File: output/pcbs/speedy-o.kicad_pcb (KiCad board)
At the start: 2 copper layers, 172 x 125.7 mm, 97 parts

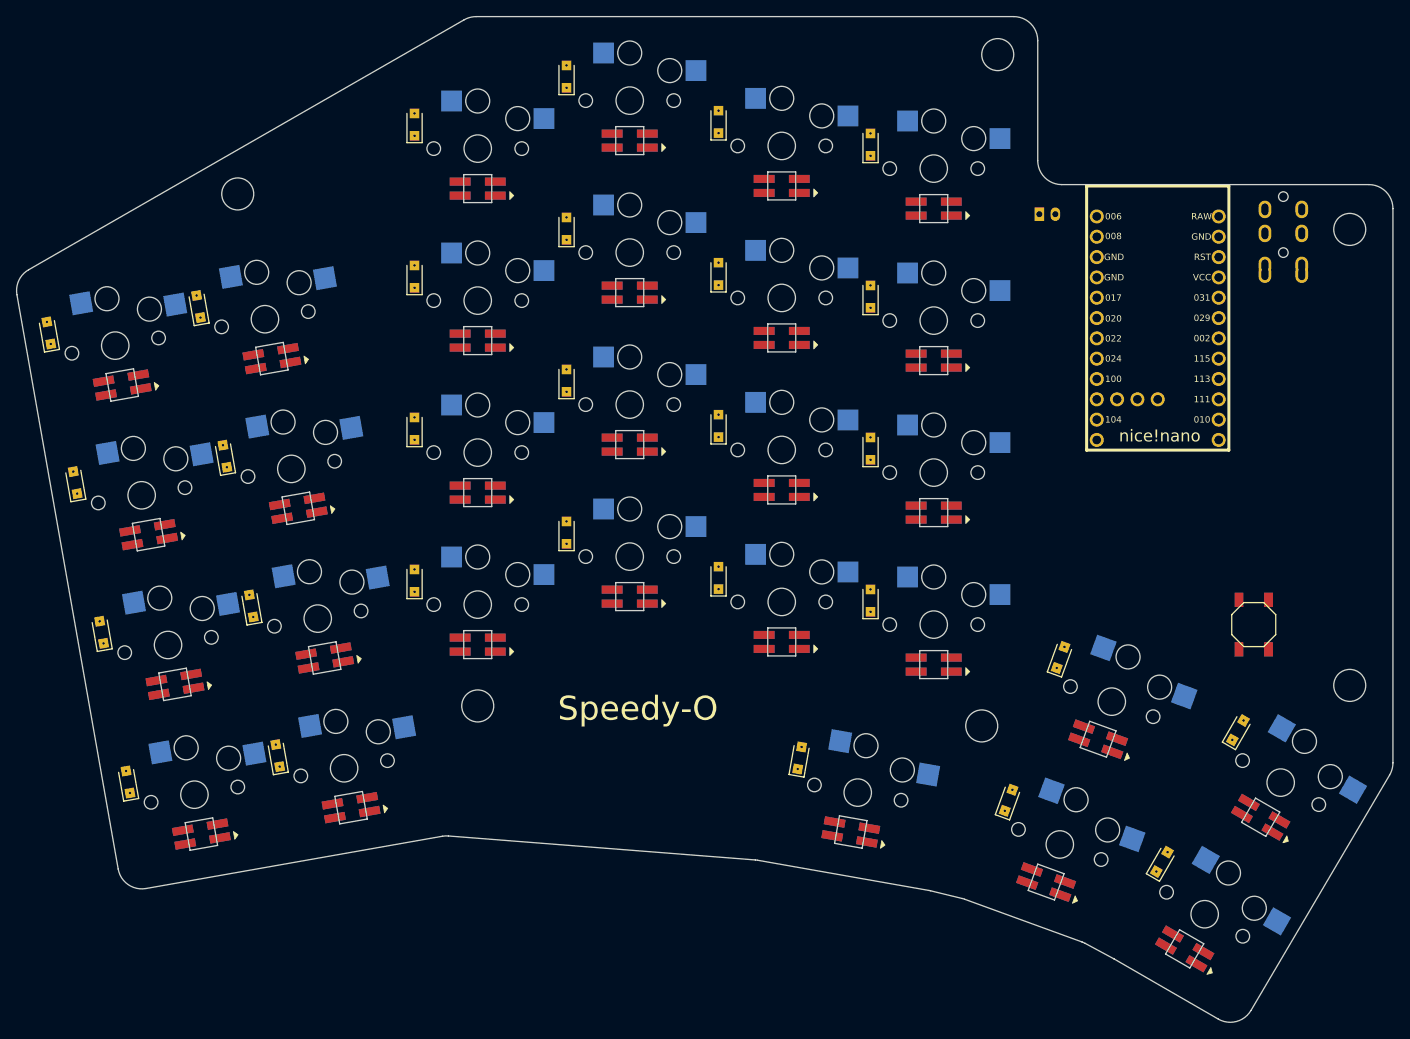
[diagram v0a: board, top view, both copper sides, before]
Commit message: update config
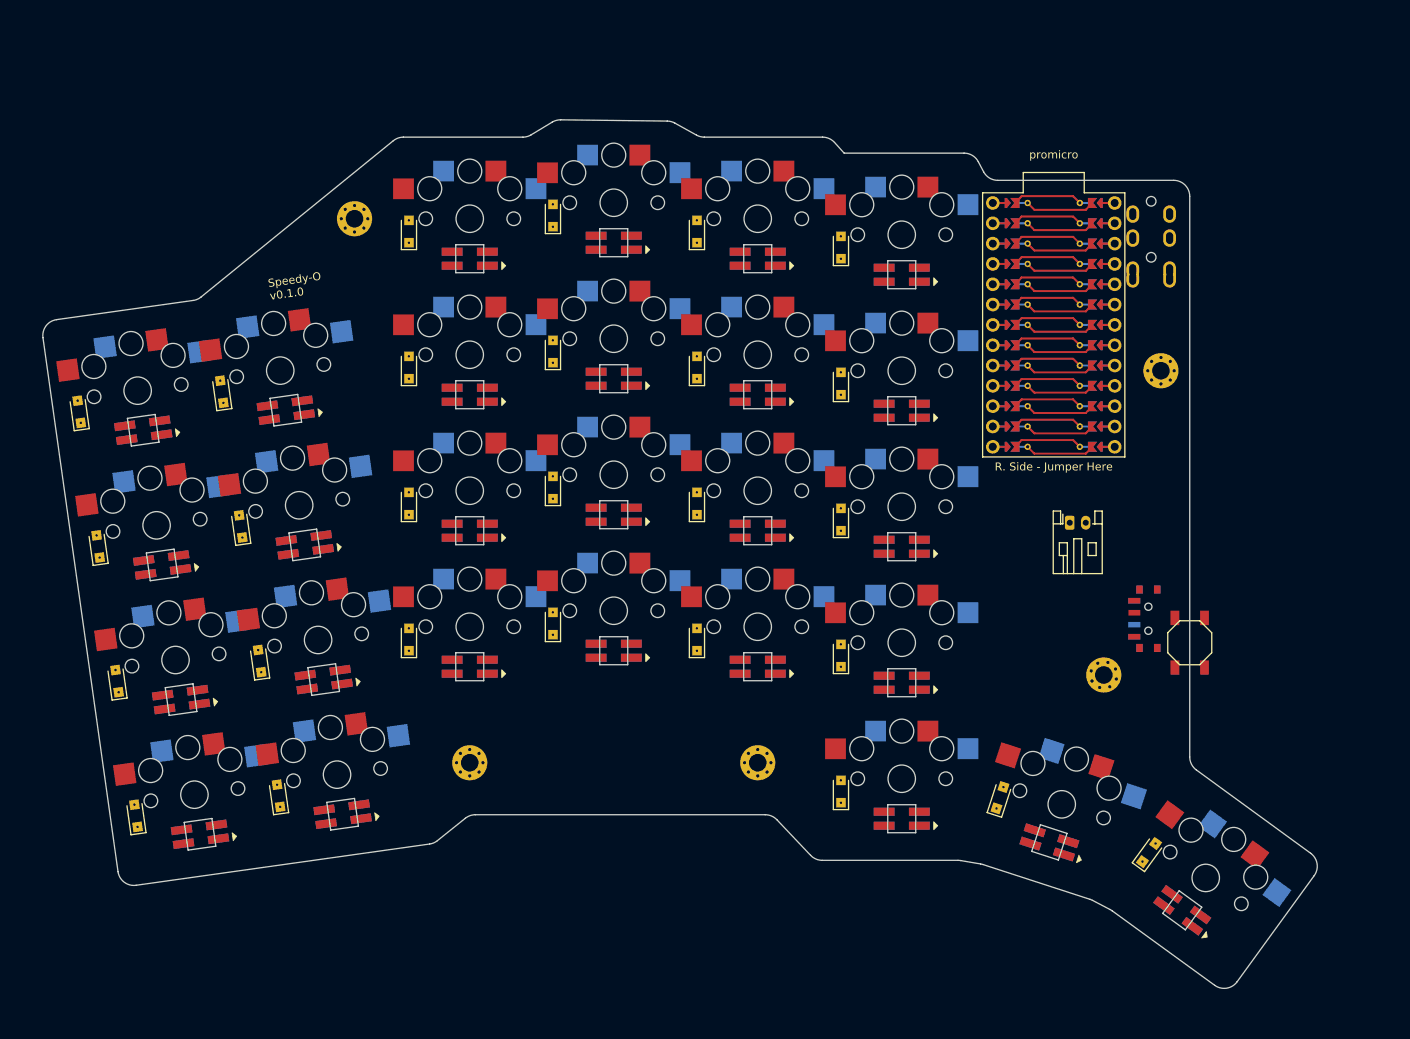
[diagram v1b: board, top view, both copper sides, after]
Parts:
- removed the ? at (135.4, 138.9)
- removed the ? at (198.4, 141.4)
- removed the ? at (244.4, 136.3)
- removed the ? at (105.4, 74.9)
- removed the ? at (200.4, 57.5)
- removed the ? at (244.4, 79.3)
- removed D28, D29: Nexperia_CFP3_SOD-123W, Diode_SMD:Nexperia_CFP3_SOD-123W
- removed JST1: , JST_PH_S2B-PH-K_02x2.00mm_Angled
- removed LED28, LED29: , WS2812B
- removed MCU1: nice_nano, nice_nano
- removed S28, S29: , PG1350
- added ?: , ProMicro, F.Cu at (207.4, 90.0)
- added T1: , Button_Switch_SMD:SW_SPDT_PCM12, F.Cu at (218.9, 128.0)
- added _2: , Connector_JST:JST_PH_S2B-PH-K_1x02_P2.00mm_Horizontal,  at (209.4, 116.0)
- added _3: , MountingHole_2.2mm_M2_Pad_Via, F.Cu at (120.0, 78.0)
- added _4: , MountingHole_2.2mm_M2_Pad_Via, F.Cu at (134.4, 146.0)
- added _5: , MountingHole_2.2mm_M2_Pad_Via, F.Cu at (170.4, 146.0)
- added _6: , MountingHole_2.2mm_M2_Pad_Via, F.Cu at (213.7, 135.0)
- added _7: , MountingHole_2.2mm_M2_Pad_Via, F.Cu at (220.8, 97.0)
- moved D27 26.8 mm to (219.3, 157.2), turned to 54 degrees
- moved S27 25.0 mm to (226.4, 160.4), turned to -36 degrees
- moved LED27 23.8 mm to (223.5, 164.5), turned to -36 degrees
- moved D16 17.4 mm to (144.8, 77.6)
- moved TRRS1 16.5 mm to (221.9, 74.2)
- moved D15 15.5 mm to (144.8, 94.6)
- moved D20 14.0 mm to (162.8, 79.6)
- moved D14 13.5 mm to (144.8, 111.6)
- moved D24 13.4 mm to (180.8, 81.6)
- moved D12 13.4 mm to (126.8, 79.6)
- moved LED16 12.9 mm to (152.4, 81.0)
- moved S16 12.9 mm to (152.4, 76.0)
- moved D19 12.0 mm to (162.8, 96.6)
- moved D13 11.5 mm to (144.8, 128.6)
- moved D23 11.5 mm to (180.8, 98.6)
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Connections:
- net P006 renamed P10
- net P008 renamed P9
- net P011 renamed P2
- net P017 renamed P8
- net P100 renamed P1
- net P104 renamed P3
- net P106 renamed P4
- net first_home renamed thumb_inner_home
- net index_bottom renamed main_index_bottom
- net index_home renamed main_index_home
- net index_num renamed main_index_num
- net index_top renamed main_index_top
- net inner_bottom renamed main_inner_bottom
- net inner_home renamed main_inner_home
- net inner_num renamed main_inner_num
- net inner_top renamed main_inner_top
- net middle_bottom renamed main_middle_bottom
- net middle_home renamed main_middle_home
- net middle_num renamed main_middle_num
- net middle_top renamed main_middle_top
- net outer_bottom renamed main_outer_bottom
- net outer_home renamed main_outer_home
- net outer_num renamed main_outer_num
- net outer_top renamed main_outer_top
- net pinky_bottom renamed main_pinky_bottom
- net pinky_home renamed main_pinky_home
- net pinky_num renamed main_pinky_num
- net pinky_top renamed main_pinky_top
- net ring_bottom renamed main_ring_bottom
- net ring_home renamed main_ring_home
- net ring_num renamed main_ring_num
- net ring_top renamed main_ring_top
- net second_home renamed thumb_home_home
- net second_upper renamed thumb_outer_home
- D25 pad 1: (no net) -> P11
- D26 pad 1: (no net) -> P11
- D27 pad 1: (no net) -> P11
- LED1 pad 4: (no net) -> rgb_main_outer_bottom
- LED10 pad 2: (no net) -> rgb_main_ring_bottom
- LED10 pad 4: (no net) -> rgb_main_ring_home
- LED11 pad 2: (no net) -> rgb_main_ring_home
- LED11 pad 4: (no net) -> rgb_main_ring_top
- LED12 pad 2: (no net) -> rgb_main_ring_top
- LED12 pad 4: (no net) -> rgb_main_ring_num
- LED13 pad 2: (no net) -> rgb_main_middle_home
- LED13 pad 4: (no net) -> rgb_main_middle_bottom
- LED14 pad 2: (no net) -> rgb_main_middle_top
- LED14 pad 4: (no net) -> rgb_main_middle_home
- LED15 pad 2: (no net) -> rgb_main_middle_num
- LED15 pad 4: (no net) -> rgb_main_middle_top
- LED16 pad 2: (no net) -> rgb_main_ring_num
- LED16 pad 4: (no net) -> rgb_main_middle_num
- LED17 pad 2: (no net) -> rgb_thumb_home_home
- LED17 pad 4: (no net) -> rgb_main_index_bottom
- LED18 pad 2: (no net) -> rgb_main_index_bottom
- LED18 pad 4: (no net) -> rgb_main_index_home
- LED19 pad 2: (no net) -> rgb_main_index_home
- LED19 pad 4: (no net) -> rgb_main_index_top
- LED2 pad 2: (no net) -> rgb_main_outer_bottom
- LED2 pad 4: (no net) -> rgb_main_outer_home
- LED20 pad 2: (no net) -> rgb_main_index_top
- LED20 pad 4: (no net) -> rgb_main_index_num
- LED21 pad 2: (no net) -> rgb_main_inner_home
- LED21 pad 4: (no net) -> rgb_main_inner_bottom
- LED22 pad 2: (no net) -> rgb_main_inner_top
- LED22 pad 4: (no net) -> rgb_main_inner_home
- LED23 pad 2: (no net) -> rgb_main_inner_num
- LED23 pad 4: (no net) -> rgb_main_inner_top
- LED24 pad 2: (no net) -> rgb_main_index_num
- LED24 pad 4: (no net) -> rgb_main_inner_num
- LED25 pad 2: (no net) -> rgb_main_middle_bottom
- LED25 pad 4: (no net) -> rgb_thumb_inner_home
- LED26 pad 2: (no net) -> rgb_thumb_inner_home
- LED26 pad 4: (no net) -> rgb_thumb_home_home
- LED27 pad 2: (no net) -> rgb_main_inner_bottom
- LED27 pad 4: (no net) -> P12
- LED3 pad 2: (no net) -> rgb_main_outer_home
- LED3 pad 4: (no net) -> rgb_main_outer_top
- LED4 pad 2: (no net) -> rgb_main_outer_top
- LED4 pad 4: (no net) -> rgb_main_outer_num
- LED5 pad 2: (no net) -> rgb_main_pinky_home
- LED5 pad 4: (no net) -> rgb_main_pinky_bottom
- LED6 pad 2: (no net) -> rgb_main_pinky_top
- LED6 pad 4: (no net) -> rgb_main_pinky_home
- LED7 pad 2: (no net) -> rgb_main_pinky_num
- LED7 pad 4: (no net) -> rgb_main_pinky_top
- LED8 pad 2: (no net) -> rgb_main_outer_num
- LED8 pad 4: (no net) -> rgb_main_pinky_num
- LED9 pad 2: (no net) -> rgb_main_pinky_bottom
- LED9 pad 4: (no net) -> rgb_main_ring_bottom
- S13 pad 1: P020 -> P7
- S14 pad 1: P020 -> P7
- S15 pad 1: P020 -> P7
- S16 pad 1: P020 -> P7
- S17 pad 1: P022 -> P6
- S18 pad 1: P022 -> P6
- S19 pad 1: P022 -> P6
- S20 pad 1: P022 -> P6
- S21 pad 1: P024 -> P5
- S22 pad 1: P024 -> P5
- S23 pad 1: P024 -> P5
- S24 pad 1: P024 -> P5
- S25 pad 1: P009 -> P5
- S26 pad 1: P010 -> P6
- S27 pad 1: P111 -> P7
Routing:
- net (no net): track 0.00 -> 371.4 mm
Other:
- board size 172 x 125.7 mm -> 159.3 x 108.6 mm
- board text added: "Speedy-O v0.1.0"
- board text removed: "Speedy-O"

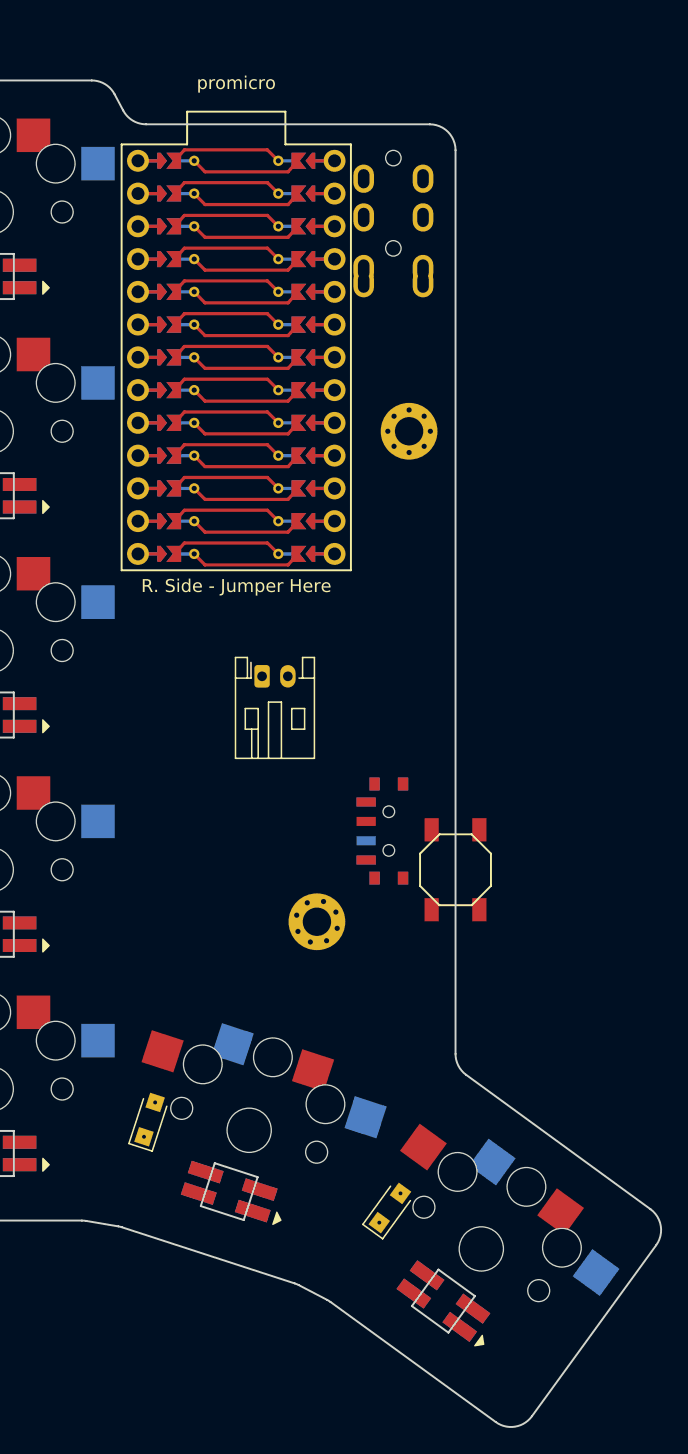
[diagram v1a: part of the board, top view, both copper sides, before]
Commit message: alternative layout
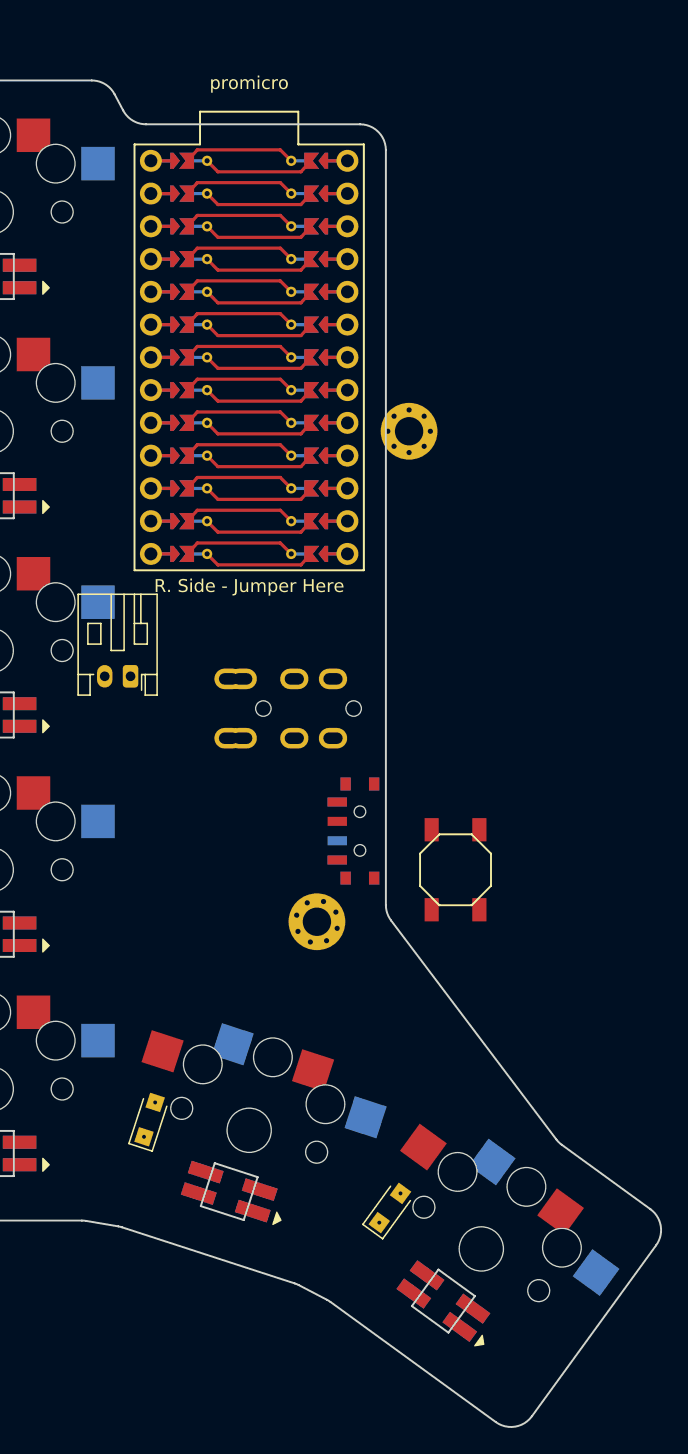
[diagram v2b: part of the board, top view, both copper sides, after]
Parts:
- moved TRRS1 46.7 mm to (218.1, 120.8), turned to -90 degrees
- moved _2 10.2 mm to (199.2, 116.0), turned to 180 degrees
- moved T1 2.24 mm to (216.7, 128.0)
- moved ? 1.00 mm to (208.4, 90.0)
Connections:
- D25 pad 1: P11 -> P8
- D25 pad 2: thumb_inner_home -> thumb_outer_home
- D26 pad 1: P11 -> P8
- D27 pad 1: P11 -> P8
- D27 pad 2: thumb_outer_home -> thumb_inner_home
- LED25 pad 4: rgb_thumb_inner_home -> rgb_thumb_outer_home
- LED27 pad 4: P12 -> P9
- S25 pad 2: thumb_inner_home -> thumb_outer_home
- S26 pad 1: P6 -> P4
- S27 pad 1: P7 -> P3
- S27 pad 2: thumb_outer_home -> thumb_inner_home
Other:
- outline, holes or cut-outs redrawn

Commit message: update routing
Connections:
- D1 pad 1: P1 -> P6
- D10 pad 1: P2 -> P7
- D11 pad 1: P3 -> P8
- D12 pad 1: P4 -> P9
- D13 pad 1: P1 -> P6
- D14 pad 1: P2 -> P7
- D15 pad 1: P3 -> P8
- D16 pad 1: P4 -> P9
- D17 pad 1: P1 -> P6
- D18 pad 1: P2 -> P7
- D19 pad 1: P3 -> P8
- D2 pad 1: P2 -> P7
- D20 pad 1: P4 -> P9
- D21 pad 1: P1 -> P6
- D22 pad 1: P2 -> P7
- D23 pad 1: P3 -> P8
- D24 pad 1: P4 -> P9
- D25 pad 1: P8 -> P16
- D26 pad 1: P8 -> P16
- D27 pad 1: P8 -> P16
- D3 pad 1: P3 -> P8
- D4 pad 1: P4 -> P9
- D5 pad 1: P1 -> P6
- D6 pad 1: P2 -> P7
- D7 pad 1: P3 -> P8
- D8 pad 1: P4 -> P9
- D9 pad 1: P1 -> P6
- LED1 pad 2: (no net) -> rgb_main_outer_home
- LED10 pad 2: rgb_main_ring_bottom -> rgb_main_pinky_top
- LED11 pad 2: rgb_main_ring_home -> rgb_main_middle_top
- LED12 pad 2: rgb_main_ring_top -> (no net)
- LED13 pad 2: rgb_main_middle_home -> rgb_main_index_bottom
- LED14 pad 2: rgb_main_middle_top -> rgb_main_ring_home
- LED15 pad 2: rgb_main_middle_num -> rgb_main_index_top
- LED17 pad 2: rgb_thumb_home_home -> rgb_main_inner_bottom
- LED18 pad 2: rgb_main_index_bottom -> rgb_main_middle_home
- LED19 pad 2: rgb_main_index_home -> rgb_main_inner_top
- LED2 pad 2: rgb_main_outer_bottom -> rgb_main_pinky_home
- LED20 pad 2: rgb_main_index_top -> rgb_main_middle_num
- LED22 pad 2: rgb_main_inner_top -> rgb_main_index_home
- LED25 pad 2: rgb_main_middle_bottom -> rgb_main_pinky_bottom
- LED26 pad 2: rgb_thumb_inner_home -> rgb_thumb_outer_home
- LED27 pad 2: rgb_main_inner_bottom -> rgb_thumb_home_home
- LED3 pad 2: rgb_main_outer_home -> rgb_main_outer_num
- LED4 pad 2: rgb_main_outer_top -> rgb_main_pinky_num
- LED5 pad 2: rgb_main_pinky_home -> rgb_main_outer_bottom
- LED6 pad 2: rgb_main_pinky_top -> rgb_main_ring_bottom
- LED7 pad 2: rgb_main_pinky_num -> rgb_main_outer_top
- LED8 pad 2: rgb_main_outer_num -> rgb_main_ring_top
- LED9 pad 2: rgb_main_pinky_bottom -> rgb_main_middle_bottom
- S1 pad 1: P10 -> P3
- S10 pad 1: P8 -> P5
- S11 pad 1: P8 -> P5
- S12 pad 1: P8 -> P5
- S13 pad 1: P7 -> P18
- S14 pad 1: P7 -> P18
- S15 pad 1: P7 -> P18
- S16 pad 1: P7 -> P18
- S17 pad 1: P6 -> P15
- S18 pad 1: P6 -> P15
- S19 pad 1: P6 -> P15
- S2 pad 1: P10 -> P3
- S20 pad 1: P6 -> P15
- S21 pad 1: P5 -> P14
- S22 pad 1: P5 -> P14
- S23 pad 1: P5 -> P14
- S24 pad 1: P5 -> P14
- S25 pad 1: P5 -> P18
- S26 pad 1: P4 -> P15
- S27 pad 1: P3 -> P14
- S3 pad 1: P10 -> P3
- S4 pad 1: P10 -> P3
- S5 pad 1: P9 -> P4
- S6 pad 1: P9 -> P4
- S7 pad 1: P9 -> P4
- S8 pad 1: P9 -> P4
- S9 pad 1: P8 -> P5
- TRRS1 pad 4: P0 -> P10
